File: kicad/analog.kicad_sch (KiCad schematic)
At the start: 42 parts, among them U402 MP2672GD-0000-Z, U403 Battery (MR-30), U501 TPS63070RNMR, U601 TPS63070RNMR

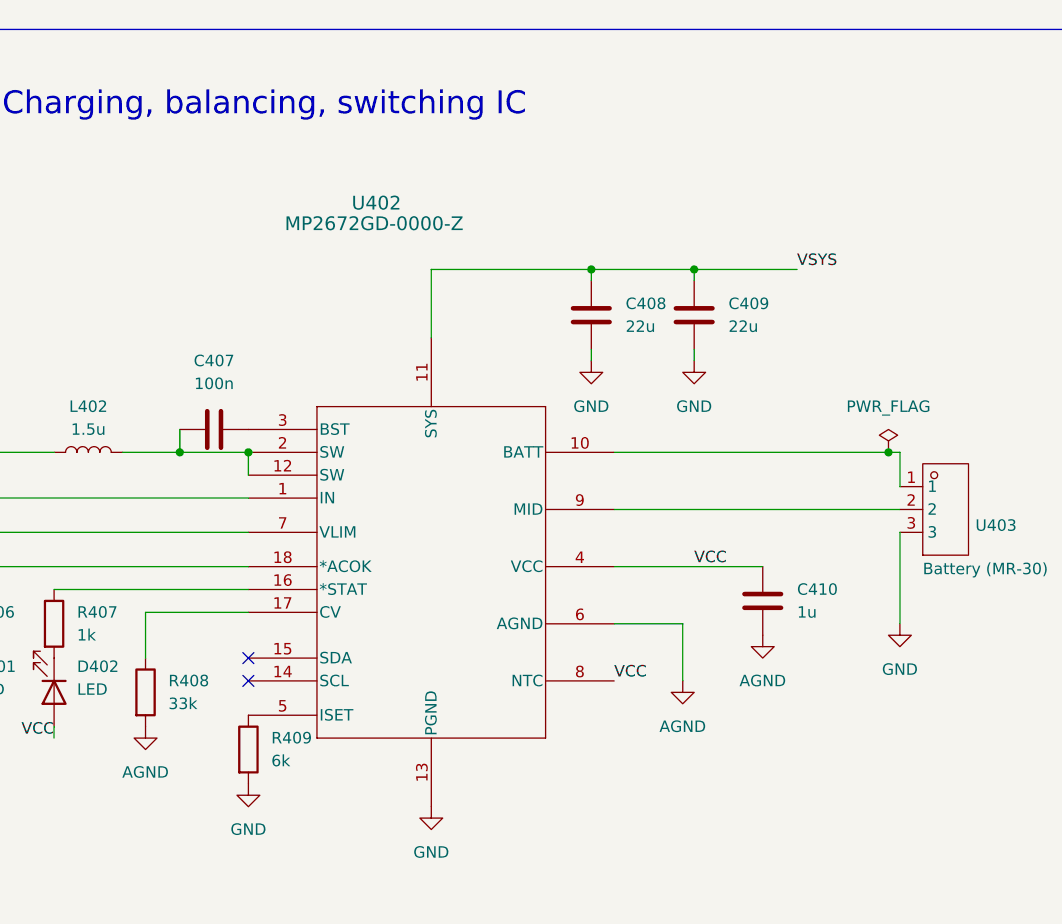
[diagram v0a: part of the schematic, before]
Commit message: export final production files for 0.1.0
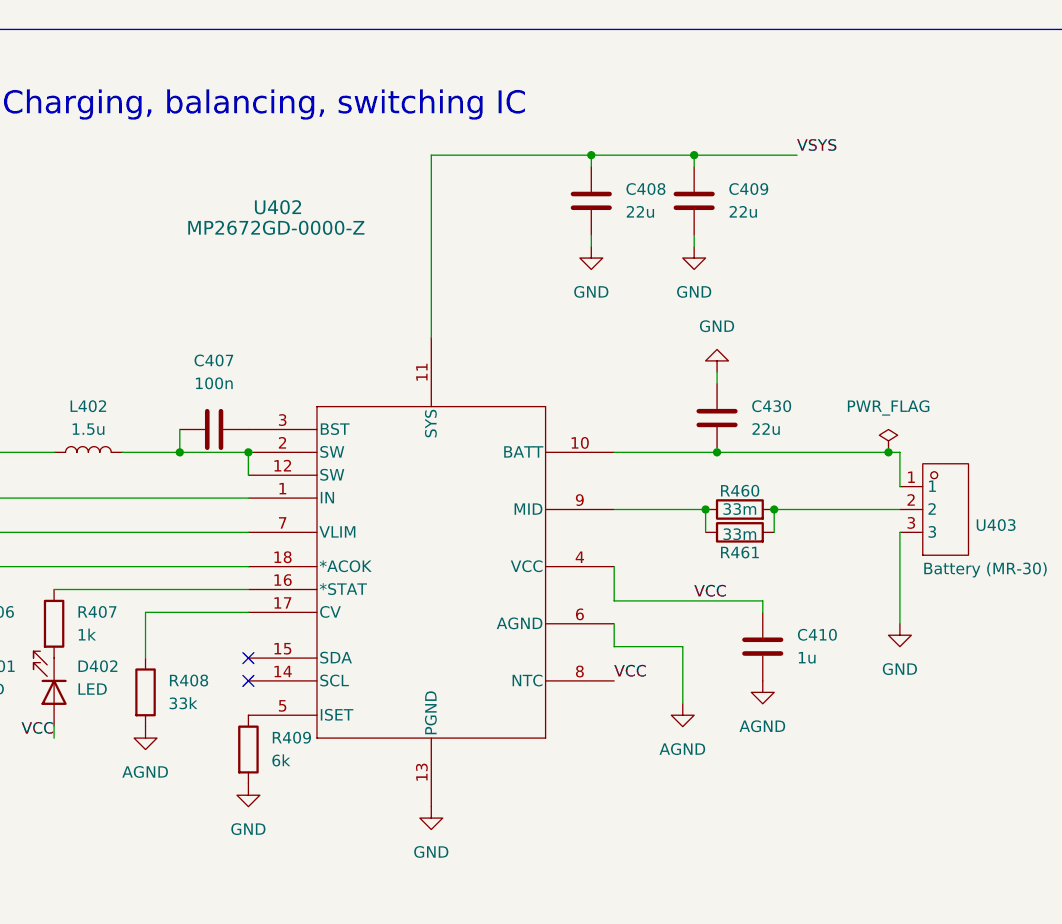
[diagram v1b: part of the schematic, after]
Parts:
- added C430: 22u, Capacitor_SMD:C_1206_3216Metric, symbol Device:C
- added R460, R461: 33m, Resistor_SMD:R_1206_3216Metric, symbol Device:R
- R503: footprint Resistor_SMD:R_0402_1005Metric -> Resistor_SMD:R_0805_2012Metric; JLC Link https://jlcpcb.com/partdetail/1518-RS02K154JT/C1166 -> https://jlcpcb.com/partdetail/18158-0805W8F1503T5E/C17470; LCSC PN C1166 -> C17470
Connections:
- net GND: now also C430.1
- net at U402.10 (BATT), U403.1: now also C430.2
- net at U402.9 (MID): now also R460.1, R461.1; no longer U403.2
- new net: R460.2, R461.2, U403.2
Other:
- moved on the sheet: C408, C409, C410
